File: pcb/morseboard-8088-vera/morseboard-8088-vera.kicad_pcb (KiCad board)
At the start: 2 copper layers, 174.4 x 127 mm, 62 parts, among them J1 USB_B, J2 UART1, J3 Bus, SW1 SW_SPDT, SW2 INTPORT, SW4 NMI, SW6 RESET, U1 8088, U10 74HCT273, U11 TL16C550, U12 74HC245, U13 MAX232, U14 DS1813, U2 74HCT573, U3 74HCT573, U4 74HCT245, U5 SST39SF040, U6 74HCT138, U7 74HCT02, U8 74HCT00, U9 AS6C4008-55PCN, X1 7.3728 MHz

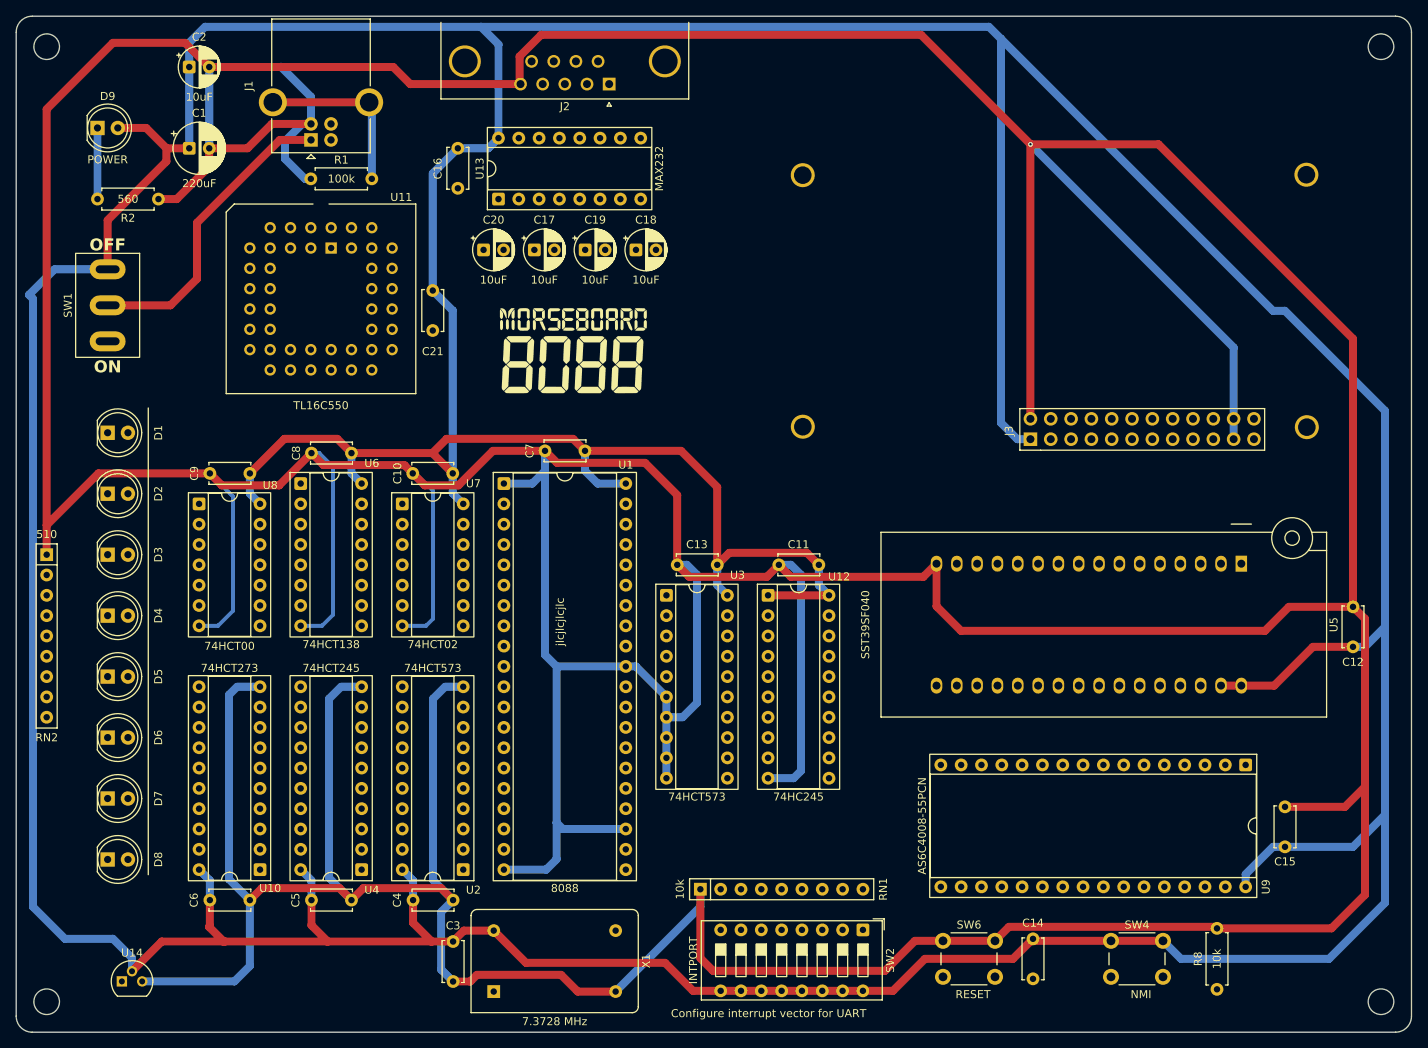
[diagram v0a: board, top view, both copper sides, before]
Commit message: Routing VERA prototype
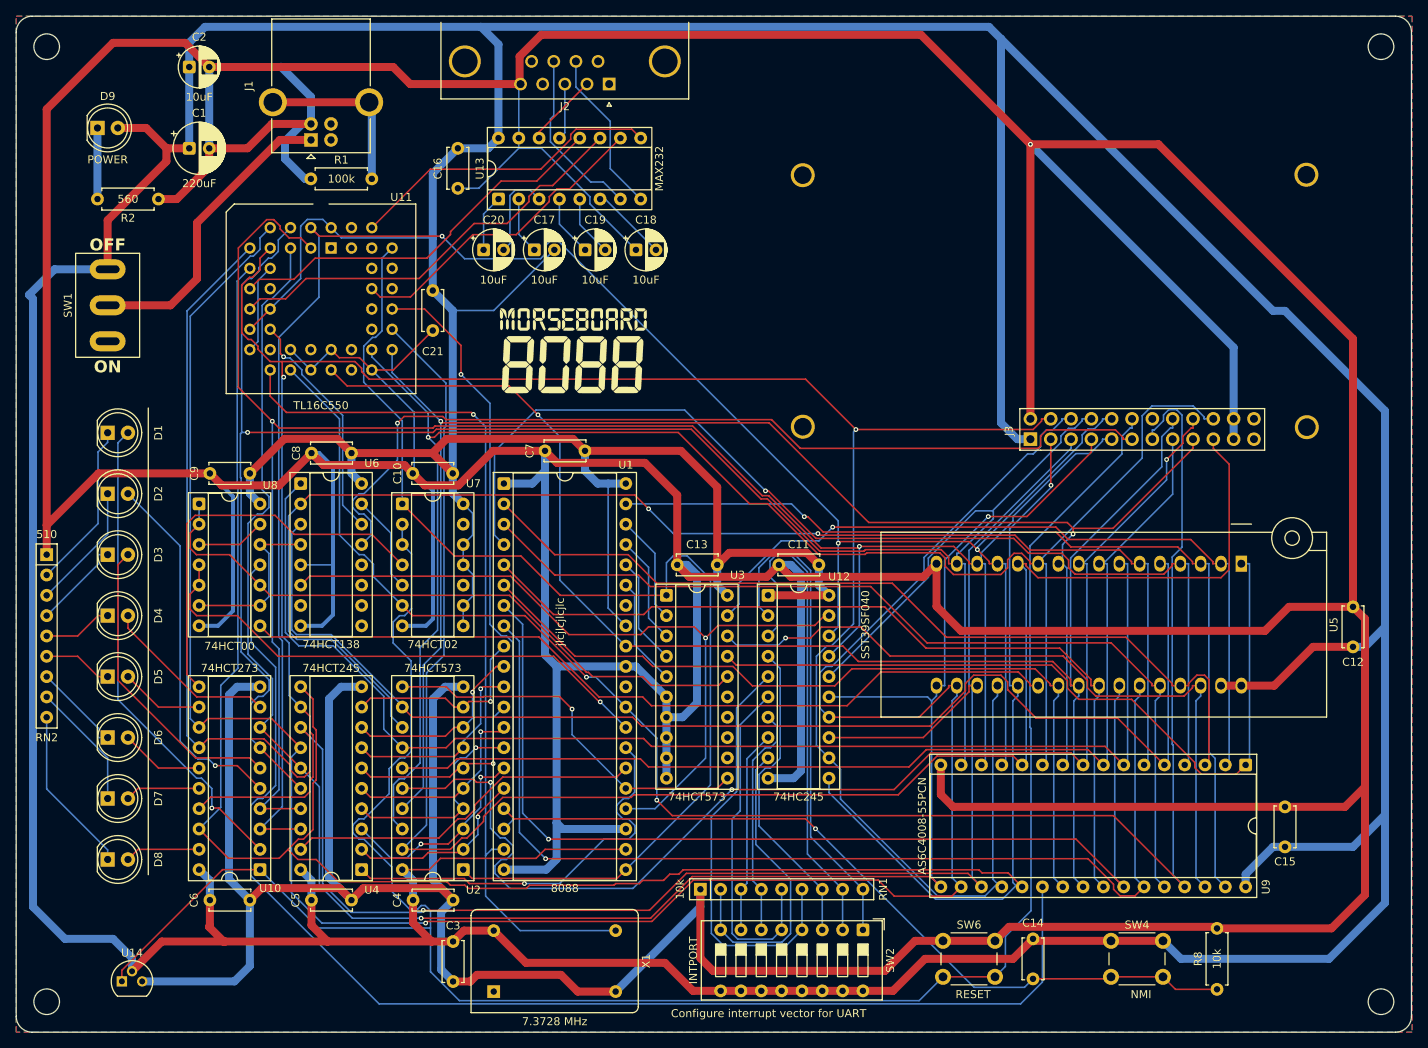
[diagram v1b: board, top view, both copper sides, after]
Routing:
- net D7: track 0.00 -> 296.1 mm, vias 0 -> 1
- net D6: track 0.00 -> 291.1 mm, vias 0 -> 2
- net D4: track 0.00 -> 285.7 mm, vias 0 -> 1
- net D5: track 0.00 -> 280.9 mm, vias 0 -> 1
- net ~{RES}: track 0.00 -> 267.1 mm
- net D2: track 0.00 -> 258.9 mm, vias 0 -> 1
- net D0: track 0.00 -> 254.6 mm, vias 0 -> 3
- net D1: track 0.00 -> 252.2 mm, vias 0 -> 2
- net D3: track 0.00 -> 251.4 mm, vias 0 -> 2
- net A0: track 0.00 -> 223.9 mm
- net ~{WR}: track 0.00 -> 219.2 mm, vias 0 -> 2
- net A1: track 0.00 -> 213.7 mm, vias 0 -> 1
- net A2: track 0.00 -> 197.8 mm, vias 0 -> 2
- net ~{RD}: track 0.00 -> 186.5 mm, vias 0 -> 1
- net A6: track 0.00 -> 172.4 mm, vias 0 -> 2
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- added copper zone on F.Cu, net GND
- added copper zone on B.Cu, net VCC
